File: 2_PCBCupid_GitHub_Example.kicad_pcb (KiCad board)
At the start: 2 copper layers, 6 parts, among them J1 Conn_01x02, SW2 SW_DPST_x2

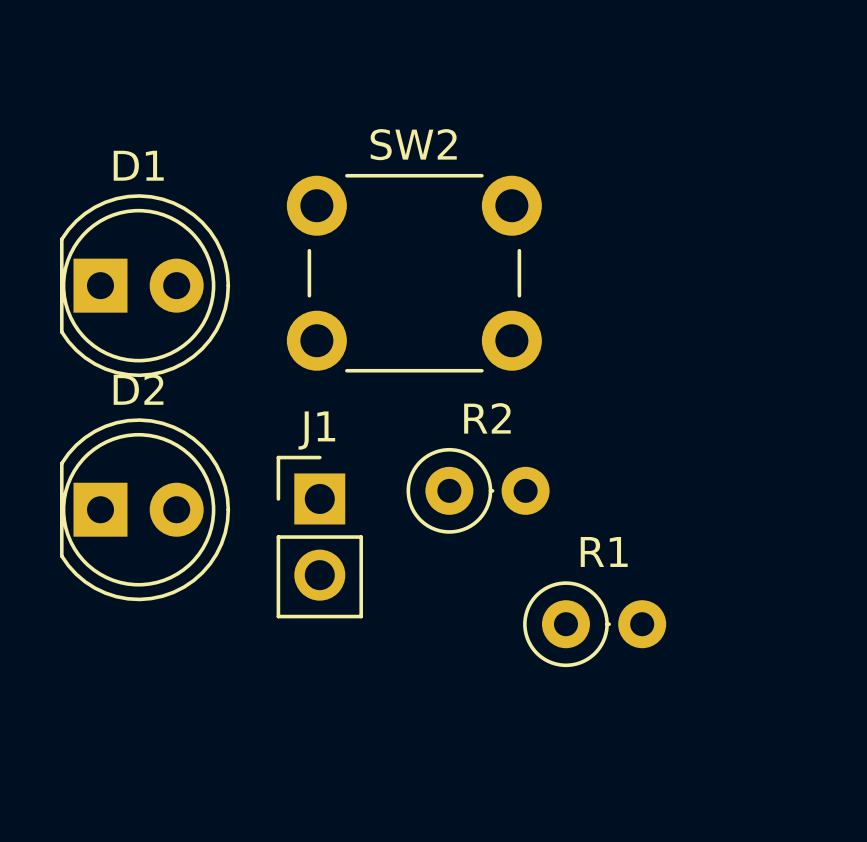
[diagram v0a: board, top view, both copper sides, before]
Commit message: Layout completed
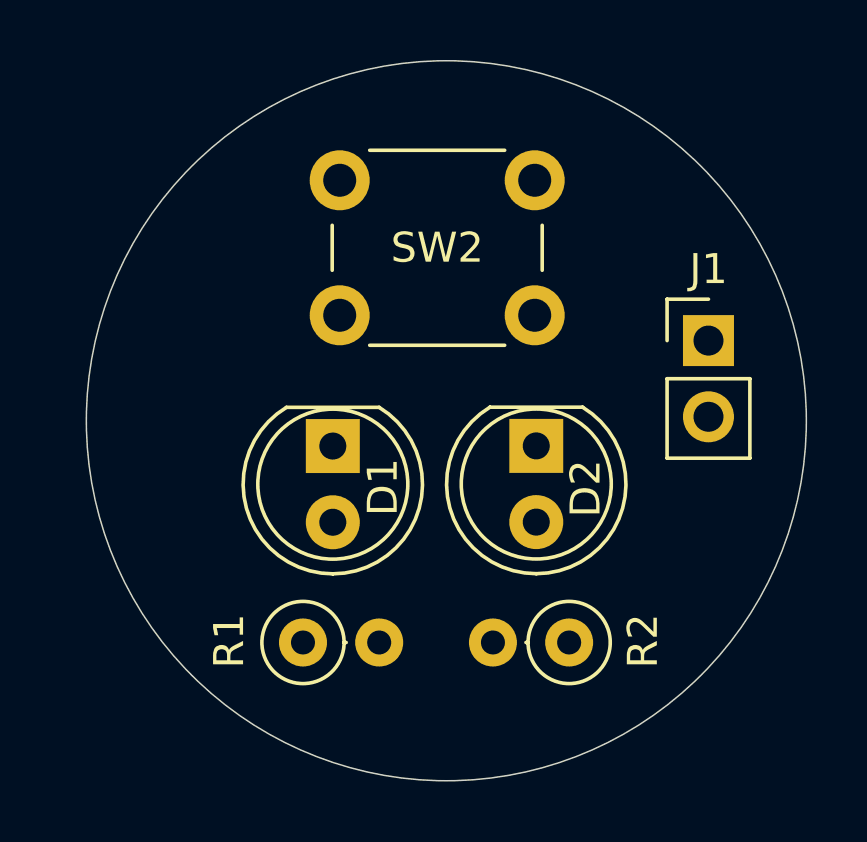
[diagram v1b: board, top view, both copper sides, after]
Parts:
- moved D2 14.7 mm to (137.1, 90.1), turned to -90 degrees
- moved J1 14.0 mm to (142.8, 86.6)
- moved D1 9.41 mm to (130.3, 90.1), turned to -90 degrees
- moved R1 8.79 mm to (129.3, 96.7)
- moved SW2 8.13 mm to (137.0, 85.8), turned to 180 degrees
- moved R2 6.44 mm to (138.2, 96.7), turned to 180 degrees
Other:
- board outline added: 24 x 24 mm
